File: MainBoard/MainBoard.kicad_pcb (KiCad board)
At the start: 4 copper layers, 34.4 x 110 mm, 42 parts, among them U1 TL074CN, U2 TL074CN, U3 TL074CN

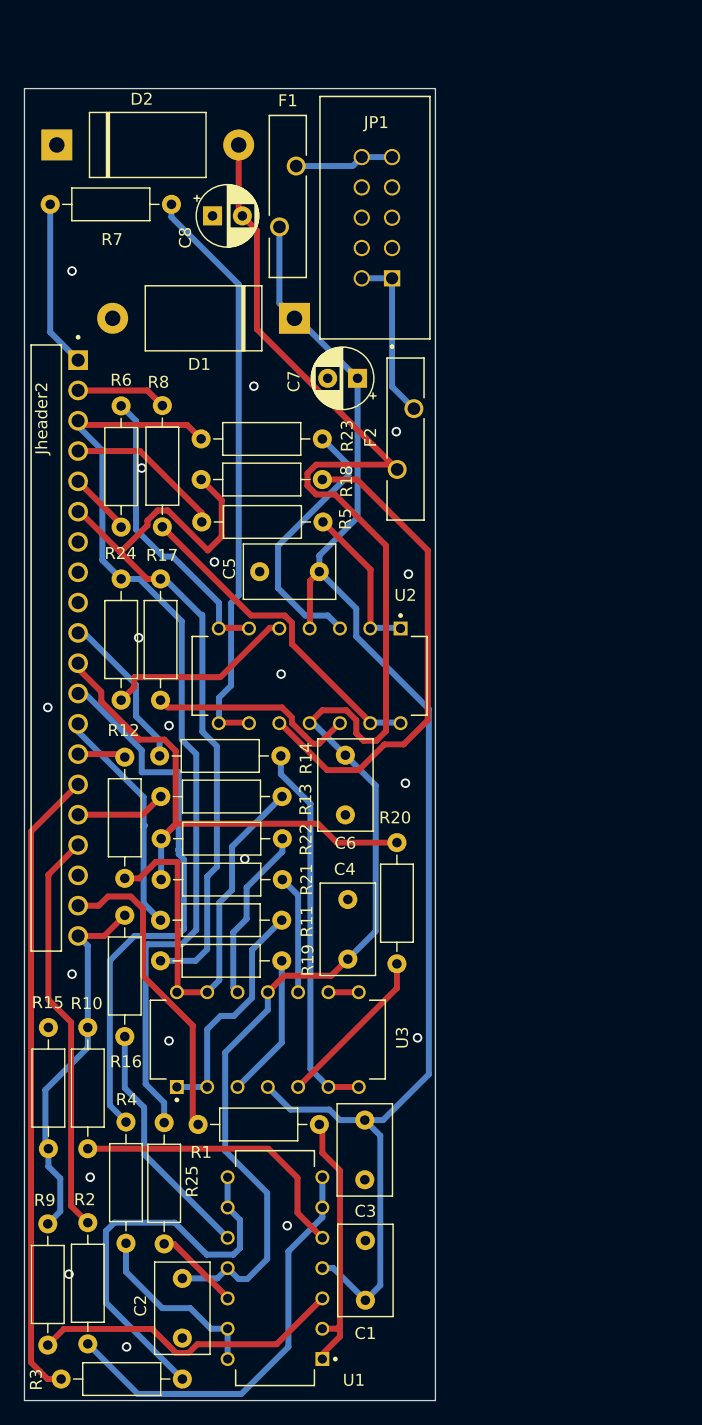
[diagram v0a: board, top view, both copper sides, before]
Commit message: sent to production v1.0.0
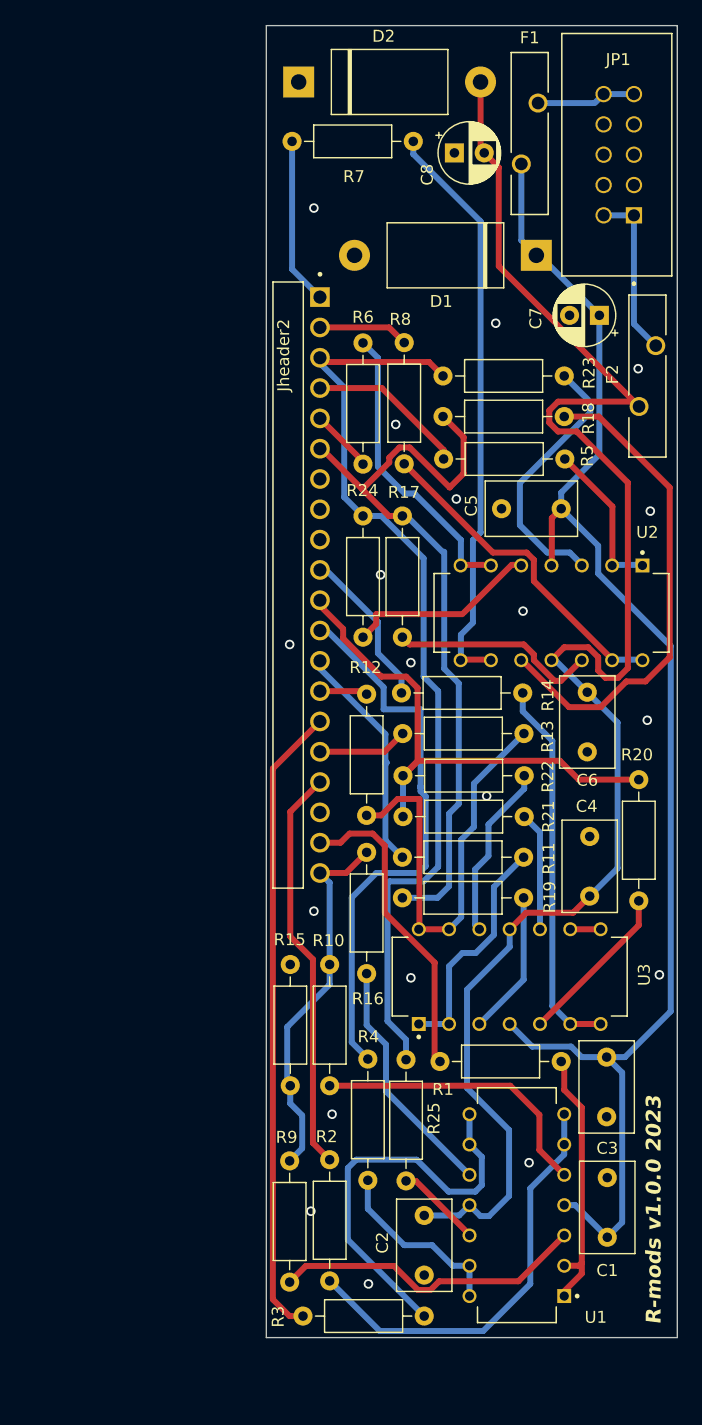
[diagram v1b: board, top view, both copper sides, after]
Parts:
- moved C1 20.9 mm to (186.6, 140.9)
- moved C2 20.9 mm to (171.2, 139.1)
- moved C5 20.9 mm to (182.7, 79.9)
- moved C6 20.9 mm to (184.9, 95.2)
- moved JP1 20.9 mm to (188.8, 55.3)
- moved Jheader2 20.9 mm to (162.5, 86.3)
- moved R1 20.9 mm to (172.6, 126.2)
- moved R10 20.9 mm to (163.3, 128.2)
- moved R11 20.9 mm to (169.4, 109.1)
- moved R14 20.9 mm to (169.3, 95.3)
- moved R15 20.9 mm to (160.0, 128.2)
- moved R16 20.9 mm to (166.4, 118.8)
- moved R18 20.9 mm to (183.0, 72.1)
- moved R19 20.9 mm to (179.6, 112.5)
- moved R23 20.9 mm to (172.8, 68.7)
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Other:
- board text added: "R-mods v1.0.0 2023"
